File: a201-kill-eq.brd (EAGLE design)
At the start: 100 x 50 mm, 86 parts, among them U10 NUT-M2-SELFLOCK, U11 FX2-20S-1.27DS, U2 SCREW-M2X8, U3 SCREW-M2X8, U4 NUT-M2-SELFLOCK, U5 NUT-M2-SELFLOCK, U6 FX2-20P-1.27DS, U7 SCREW-M2X8, U8 SCREW-M2X8, U9 NUT-M2-SELFLOCK

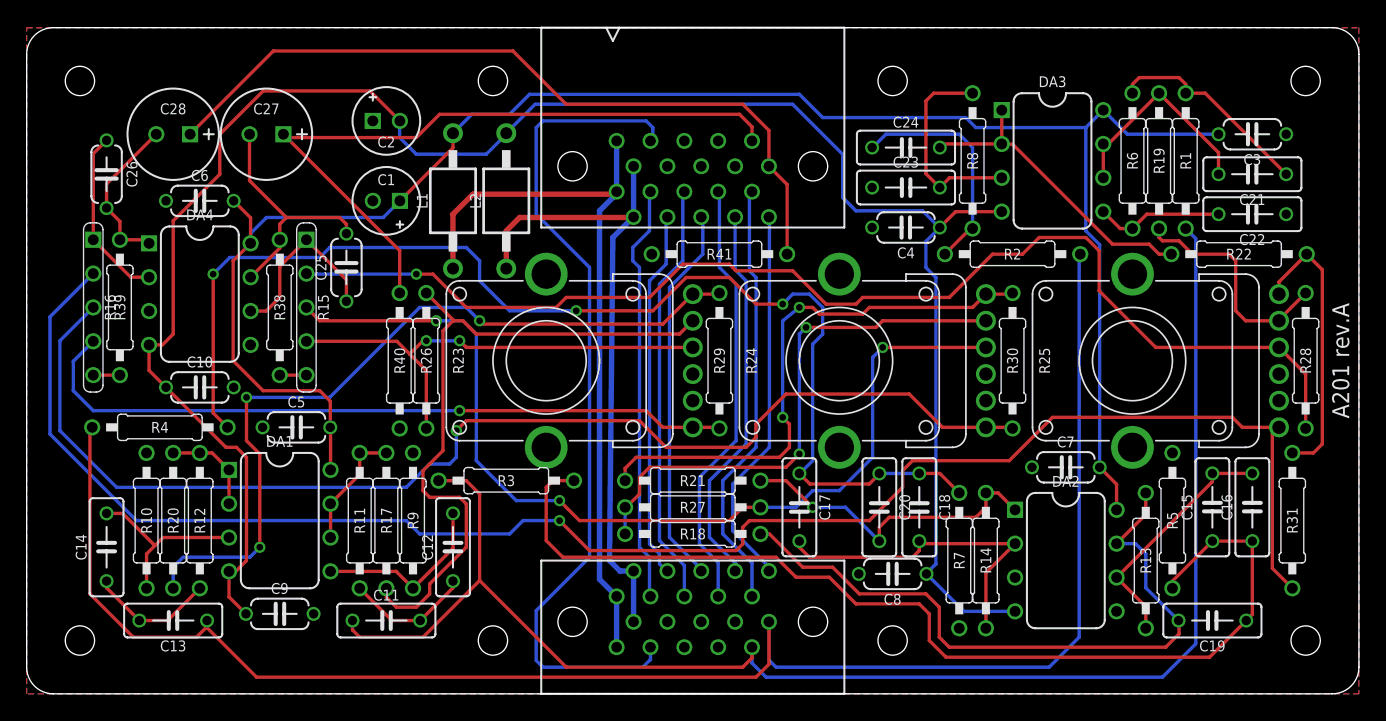
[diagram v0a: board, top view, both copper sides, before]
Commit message: PCB Update
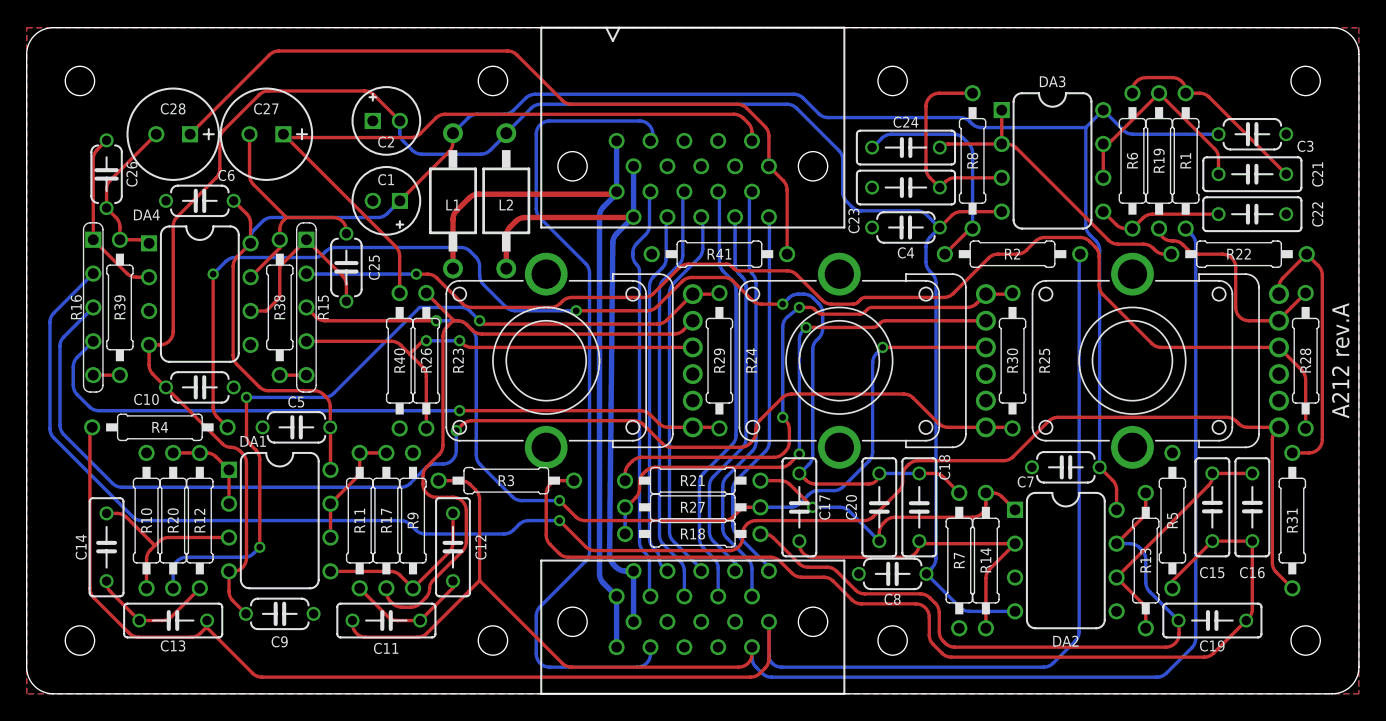
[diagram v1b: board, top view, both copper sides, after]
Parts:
- PCB1: value A201 rev.A -> A212 rev.A
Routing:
- net N$47: track 149.1 -> 147.3 mm
- net N$43: track 128.9 -> 127.2 mm
- net N$7: track 63.5 -> 62.1 mm
- net N$13: track 51.6 -> 50.3 mm
- net N$45: track 137.1 -> 135.8 mm
- net N$33: track 90.5 -> 89.2 mm
- net N$24: track 90.8 -> 89.6 mm
- net N$37: track 90.9 -> 89.8 mm
- net N$15: track 78.7 -> 77.6 mm
- net LIO: track 113.9 -> 112.9 mm
- net N$23: track 17.4 -> 16.4 mm
- net N$19: track 73.0 -> 72.2 mm
- net N$17: track 50.9 -> 50.2 mm
- net N$20: track 15.8 -> 15.2 mm
- net RIO: track 126.9 -> 126.3 mm
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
